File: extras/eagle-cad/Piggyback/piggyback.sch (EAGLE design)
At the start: 3 parts

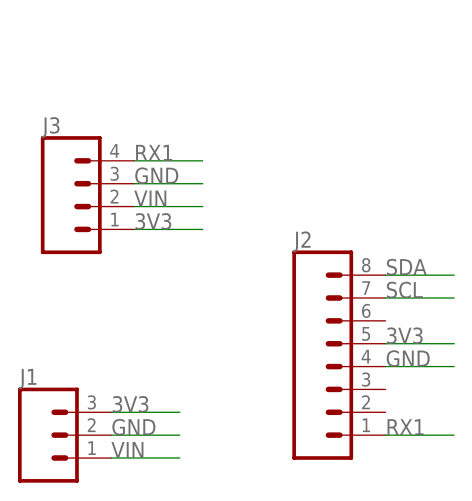
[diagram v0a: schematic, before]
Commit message: More Butterfly Piggyback board work
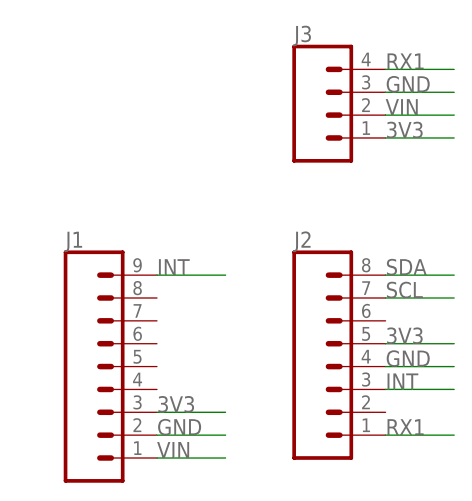
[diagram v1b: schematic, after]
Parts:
- J1: device SparkFun-Connectors:CONN_031X03_NO_SILK -> SparkFun-Connectors:CONN_09NO_SILK
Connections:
- new net INT: J1.9, J2.3
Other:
- moved on the sheet: J3
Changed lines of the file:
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@@
 <?xml version="1.0" encoding="utf-8"?>
 <!DOCTYPE eagle SYSTEM "eagle.dtd">
-<eagle version="9.6.2">
+<eagle version="9.1.1">
 <drawing>
 <settings>
@@
 </classes>
 <parts>
-<part name="J1" library="SparkFun-Connectors" deviceset="CONN_03" device="1X03_NO_SILK"/>
 <part name="J2" library="SparkFun-Connectors" deviceset="CONN_08" device="NO_SILK_FEMALE_PTH"/>
 <part name="J3" library="SparkFun-Connectors" deviceset="CONN_04" device="1X04_NO_SILK"/>
+<part name="J1" library="SparkFun-Connectors" deviceset="CONN_09" device="NO_SILK"/>
 </parts>
 <sheets>
@@
 </plain>
 <instances>
-<instance part="J1" gate="J$1" x="-119.38" y="-2.54" smashed="yes">
-<attribute name="VALUE" x="-121.92" y="-9.906" size="1.778" layer="96" font="vector"/>
-<attribute name="NAME" x="-121.92" y="3.048" size="1.778" layer="95" font="vector"/>
-</instance>
 <instance part="J2" gate="G$1" x="-86.36" y="5.08" smashed="yes">
 <attribute name="VALUE" x="-91.44" y="-7.366" size="1.778" layer="96" font="vector"/>
 <attribute name="NAME" x="-91.44" y="18.288" size="1.778" layer="95" font="vector"/>
 </instance>
-<instance part="J3" gate="J1" x="-114.3" y="22.86" smashed="yes">
-<attribute name="VALUE" x="-119.38" y="15.494" size="1.778" layer="96" font="vector"/>
-<attribute name="NAME" x="-119.38" y="30.988" size="1.778" layer="95" font="vector"/>
+<instance part="J3" gate="J1" x="-86.36" y="33.02" smashed="yes">
+<attribute name="VALUE" x="-91.44" y="25.654" size="1.778" layer="96" font="vector"/>
+<attribute name="NAME" x="-91.44" y="41.148" size="1.778" layer="95" font="vector"/>
 </instance>
+<instance part="J1" gate="J1" x="-116.84" y="5.08"/>
 </instances>
 <busses>
@@
 <net name="VIN" class="0">
 <segment>
-<pinref part="J1" gate="J$1" pin="1"/>
-<wire x1="-111.76" y1="-5.08" x2="-104.14" y2="-5.08" width="0.1524" layer="91"/>
-<label x="-111.76" y="-5.08" size="1.778" layer="95"/>
-</segment>
-<segment>
 <pinref part="J3" gate="J1" pin="2"/>
-<wire x1="-109.22" y1="22.86" x2="-101.6" y2="22.86" width="0.1524" layer="91"/>
-<label x="-109.22" y="22.86" size="1.778" layer="95"/>
+<wire x1="-81.28" y1="33.02" x2="-73.66" y2="33.02" width="0.1524" layer="91"/>
+<label x="-81.28" y="33.02" size="1.778" layer="95"/>
+</segment>
+<segment>
+<pinref part="J1" gate="J1" pin="1"/>
+<wire x1="-106.68" y1="-5.08" x2="-99.06" y2="-5.08" width="0.1524" layer="91"/>
+<label x="-106.68" y="-5.08" size="1.778" layer="95"/>
 </segment>
 </net>
 <net name="GND" class="0">
-<segment>
-<pinref part="J1" gate="J$1" pin="2"/>
-<wire x1="-111.76" y1="-2.54" x2="-104.14" y2="-2.54" width="0.1524" layer="91"/>
-<label x="-111.76" y="-2.54" size="1.778" layer="95"/>
-</segment>
 <segment>
 <pinref part="J2" gate="G$1" pin="4"/>
@@
 <segment>
 <pinref part="J3" gate="J1" pin="3"/>
-<wire x1="-109.22" y1="25.4" x2="-101.6" y2="25.4" width="0.1524" layer="91"/>
-<label x="-109.22" y="25.4" size="1.778" layer="95"/>
+<wire x1="-81.28" y1="35.56" x2="-73.66" y2="35.56" width="0.1524" layer="91"/>
+<label x="-81.28" y="35.56" size="1.778" layer="95"/>
+</segment>
+<segment>
+<pinref part="J1" gate="J1" pin="2"/>
+<wire x1="-106.68" y1="-2.54" x2="-99.06" y2="-2.54" width="0.1524" layer="91"/>
+<label x="-106.68" y="-2.54" size="1.778" layer="95"/>
 </segment>
 </net>
 <net name="3V3" class="0">
-<segment>
-<pinref part="J1" gate="J$1" pin="3"/>
-<wire x1="-111.76" y1="0" x2="-104.14" y2="0" width="0.1524" layer="91"/>
-<label x="-111.76" y="0" size="1.778" layer="95"/>
-</segment>
 <segment>
 <pinref part="J2" gate="G$1" pin="5"/>
@@
 <segment>
 <pinref part="J3" gate="J1" pin="1"/>
-<wire x1="-109.22" y1="20.32" x2="-101.6" y2="20.32" width="0.1524" layer="91"/>
-<label x="-109.22" y="20.32" size="1.778" layer="95"/>
+<wire x1="-81.28" y1="30.48" x2="-73.66" y2="30.48" width="0.1524" layer="91"/>
+<label x="-81.28" y="30.48" size="1.778" layer="95"/>
+</segment>
+<segment>
+<pinref part="J1" gate="J1" pin="3"/>
+<wire x1="-106.68" y1="0" x2="-99.06" y2="0" width="0.1524" layer="91"/>
+<label x="-106.68" y="0" size="1.778" layer="95"/>
 </segment>
 </net>
@@
 <segment>
 <pinref part="J3" gate="J1" pin="4"/>
-<wire x1="-109.22" y1="27.94" x2="-101.6" y2="27.94" width="0.1524" layer="91"/>
-<label x="-109.22" y="27.94" size="1.778" layer="95"/>
+<wire x1="-81.28" y1="38.1" x2="-73.66" y2="38.1" width="0.1524" layer="91"/>
+<label x="-81.28" y="38.1" size="1.778" layer="95"/>
 </segment>
 </net>
@@
 </segment>
 </net>
+<net name="INT" class="0">
+<segment>
+<pinref part="J2" gate="G$1" pin="3"/>
+<wire x1="-81.28" y1="2.54" x2="-73.66" y2="2.54" width="0.1524" layer="91"/>
+<label x="-81.28" y="2.54" size="1.778" layer="95"/>
+</segment>
+<segment>
+<pinref part="J1" gate="J1" pin="9"/>
+<wire x1="-106.68" y1="15.24" x2="-99.06" y2="15.24" width="0.1524" layer="91"/>
+<label x="-106.68" y="15.24" size="1.778" layer="95"/>
+</segment>
+</net>
